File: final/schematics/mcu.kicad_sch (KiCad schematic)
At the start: 3 parts, among them U3 XIAO_ESP32C3

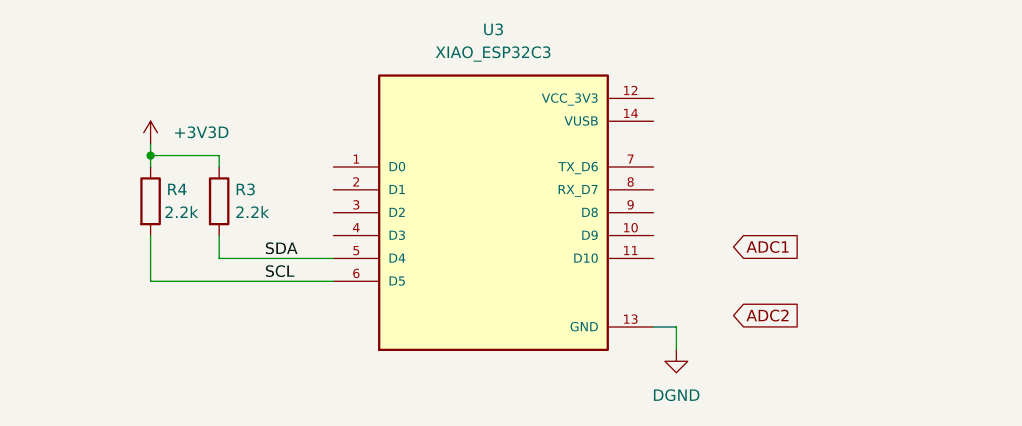
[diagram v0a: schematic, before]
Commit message: finishing
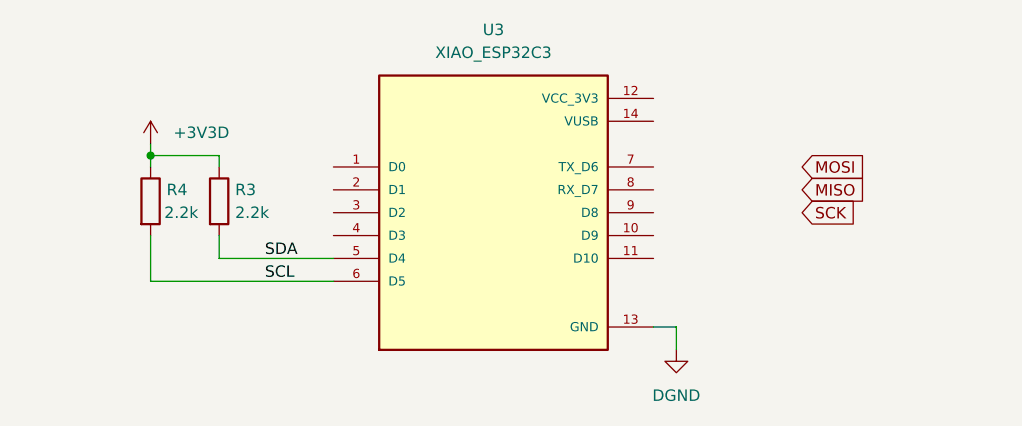
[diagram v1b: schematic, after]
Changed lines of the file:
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@@
 		)
 	)
-	(global_label "ADC2"
+	(global_label "MISO"
 		(shape input)
-		(at 151.13 87.63 0)
+		(at 158.75 73.66 0)
 		(fields_autoplaced yes)
 		(effects
@@
 		)
 		(property "Intersheetrefs" "${INTERSHEET_REFS}"
-			(at 158.9533 87.63 0)
+			(at 166.3314 73.66 0)
 			(hide yes)
 			(show_name no)
@@
 		)
 	)
-	(global_label "ADC1"
+	(global_label "MOSI"
 		(shape input)
-		(at 151.13 80.01 0)
+		(at 158.75 71.12 0)
 		(fields_autoplaced yes)
 		(effects
@@
 		)
 		(property "Intersheetrefs" "${INTERSHEET_REFS}"
-			(at 158.9533 80.01 0)
+			(at 166.3314 71.12 0)
 			(hide yes)
 			(show_name no)
+			(do_not_autoplace no)
+			(effects
+				(font
+					(size 1.27 1.27)
+				)
+				(justify left)
+			)
+		)
+	)
+	(global_label "SCK"
+		(shape input)
+		(at 158.75 76.2 0)
+		(fields_autoplaced yes)
+		(effects
+			(font
+				(size 1.27 1.27)
+			)
+			(justify left)
+		)
+		(property "Intersheetrefs" "${INTERSHEET_REFS}"
+			(at 165.4847 76.2 0)
+			(hide yes)
+			(show_name no)

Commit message: finished
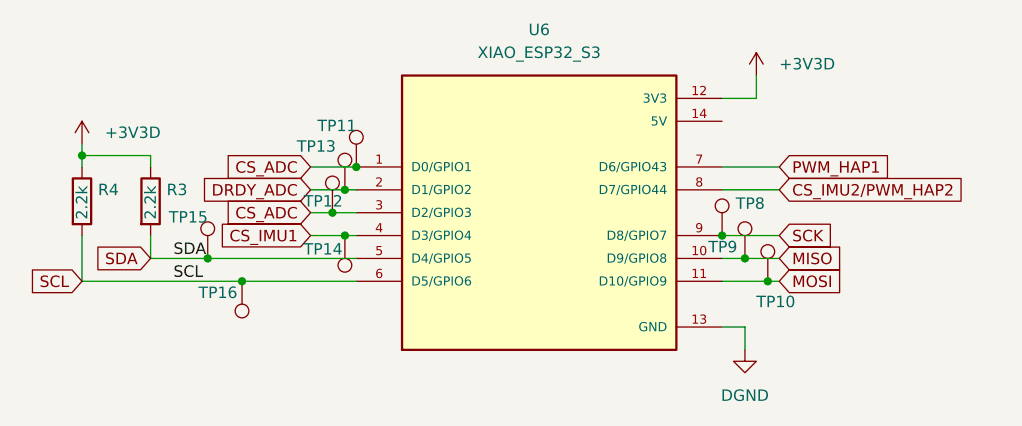
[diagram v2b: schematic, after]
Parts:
- removed U3: XIAO_ESP32C3, XIAO_ESP32C3:MODULE_XIAO_ESP32C3, symbol XIAO_ESP32C3:XIAO_ESP32C3
- added TP10, TP11, TP12, TP13, TP14, TP15, TP16, TP8, TP9: TestPoint, Connector_Pin:Pin_D1.0mm_L10.0mm_LooseFit, symbol Connector:TestPoint
- added U6: XIAO_ESP32_S3, XIAO_ESP32_S3:MODULE_XIAO_ESP32_S3, symbol XIAO_ESP32_S3:XIAO_ESP32_S3
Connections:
- net +3V3D: now also U6.12 (3V3)
- net DGND: now also U6.13 (GND)
- net MISO: now also TP9.1, U6.10 (D9/GPIO8)
- net MOSI: now also TP10.1, U6.11 (D10/GPIO9)
- net SCK: now also TP8.1, U6.9 (D8/GPIO7)
- net SCL: now also TP16.1, U6.6 (D5/GPIO6)
- net SDA: now also TP15.1, U6.5 (D4/GPIO5)
- new net CS_ADC: TP11.1, TP12.1, U6.1 (D0/GPIO1), U6.3 (D2/GPIO3)
- new net CS_IMU1: TP14.1, U6.4 (D3/GPIO4)
- new net CS_IMU2/PWM_HAP2: U6.8 (D7/GPIO44)
- new net DRDY_ADC: TP13.1, U6.2 (D1/GPIO2)
- new net PWM_HAP1: U6.7 (D6/GPIO43)
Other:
- moved on the sheet: R3, R4
